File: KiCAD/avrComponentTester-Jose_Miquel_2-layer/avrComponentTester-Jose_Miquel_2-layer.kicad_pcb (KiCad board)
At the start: 2 copper layers, 17 parts, among them J4 3-pin_test_header, Q1 2N3904, Q2 2N3904, Q3 2N3906, SW1 EC11, U1 ST7735_1.8, U2 ATmega328P-PU

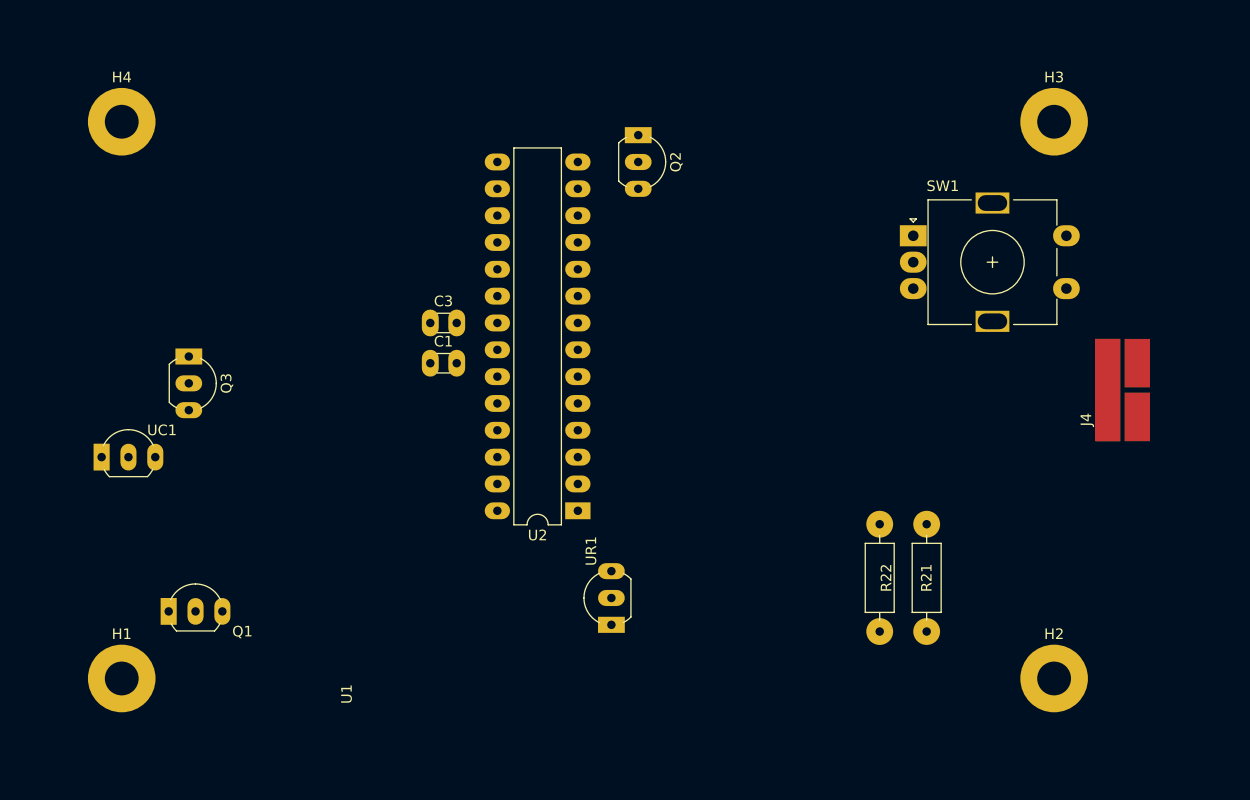
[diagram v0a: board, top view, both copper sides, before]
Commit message: kicad6
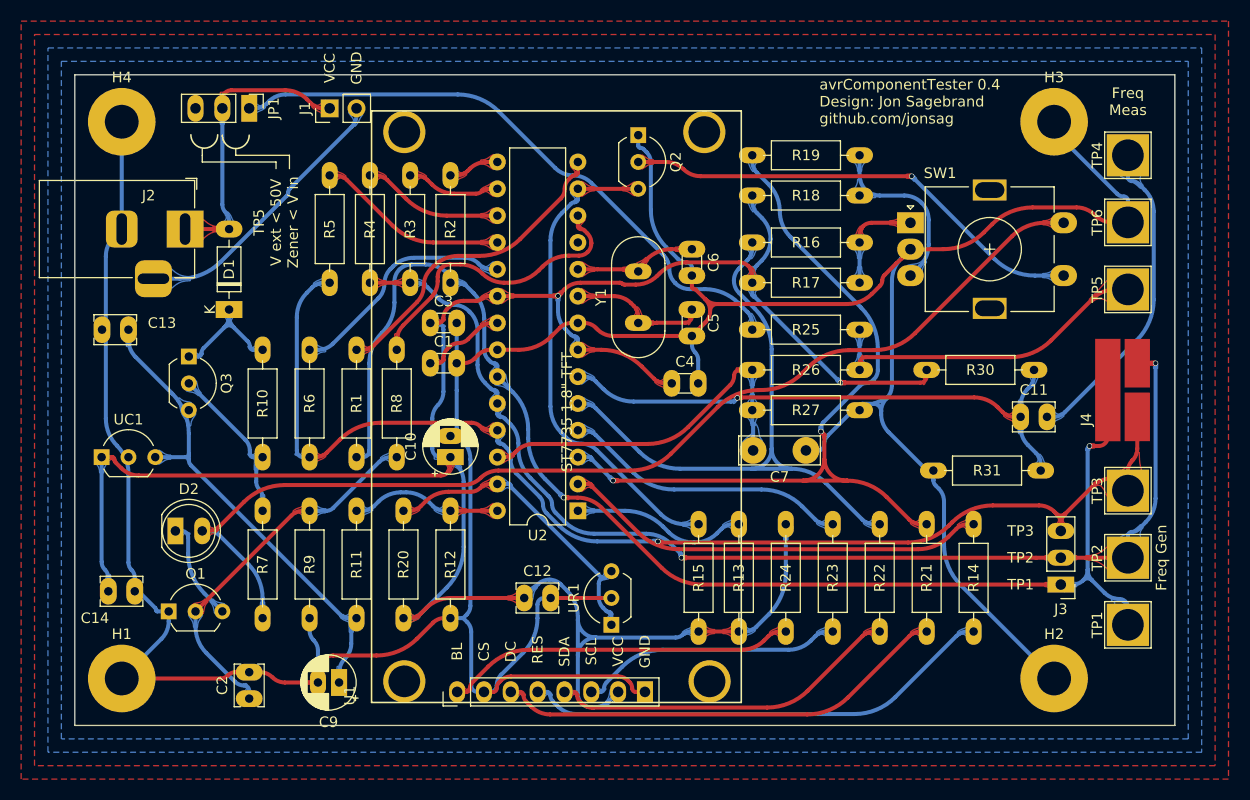
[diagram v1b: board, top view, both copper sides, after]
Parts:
- added C10: 10u, My_Misc:CP_Radial_D5.0mm_P2.00mm_larger, F.Cu at (132.7, 81.3)
- added C11: 100n, My_Misc:C_Disc_D3.8mm_W2.6mm_P2.50mm_large, F.Cu at (186.7, 77.5)
- added C12: 100n, My_Misc:C_Disc_D3.8mm_W2.6mm_P2.50mm_large, F.Cu at (139.7, 94.6)
- added C13: 100n, My_Misc:C_Disc_D3.8mm_W2.6mm_P2.50mm_large, F.Cu at (102.2, 69.2)
- added C14: 100n, My_Misc:C_Disc_D3.8mm_W2.6mm_P2.50mm_large, F.Cu at (100.3, 94.0)
- added C2: 10n, My_Misc:C_Disc_D3.8mm_W2.6mm_P2.50mm_large, F.Cu at (113.7, 104.1)
- added C4: 100n, My_Misc:C_Disc_D3.0mm_W1.6mm_P2.50mm_larg, F.Cu at (153.7, 74.3)
- added C5: 22p, My_Misc:C_Disc_D3.0mm_W1.6mm_P2.50mm_larg, F.Cu at (155.6, 67.3)
- added C6: 22p, My_Misc:C_Disc_D3.0mm_W1.6mm_P2.50mm_larg, F.Cu at (155.6, 61.6)
- added C7: 10n 100V, My_Misc:C_Disc_D7.5mm_W2.5mm_P5.00mm_larger, F.Cu at (166.4, 80.6)
- added C9: 10u, My_Misc:CP_Radial_D5.0mm_P2.00mm_larger, F.Cu at (122.2, 102.6)
- added D1: BAT43, My_Misc:D_DO-35_SOD27_P7.62mm_Horizontal_large, F.Cu at (111.8, 67.3)
- added D2: LED, My_Misc:LED_D5.0mm_larger_pads, F.Cu at (106.7, 88.3)
- added J1: 2-pin_power_input_header, My_Headers:2-pin_power_input_header, F.Cu at (121.3, 48.3)
- added J2: 8-15VDC In, My_Misc:BarrelJack_Horizontal, F.Cu at (107.6, 59.7)
- added J3: 3-pin_test_header, My_Headers:3-pin_test_header_large, F.Cu at (190.5, 93.3)
- added JP1: Vext <50V, Zener < VCC, My_Parts:Jumper_1x03_P2.54mm_large, F.Cu at (113.7, 48.3)
- added R1: 680R, My_Misc:R_Axial_DIN0207_L6.3mm_D2.5mm_P10.16mm_Horizontal_larger_pads, F.Cu at (123.8, 71.1)
- added R10: 33k, My_Misc:R_Axial_DIN0207_L6.3mm_D2.5mm_P10.16mm_Horizontal_larger_pads, F.Cu at (114.9, 81.3)
- added R11: 10k, My_Misc:R_Axial_DIN0207_L6.3mm_D2.5mm_P10.16mm_Horizontal_larger_pads, F.Cu at (123.8, 96.5)
- added R12: 3k3, My_Misc:R_Axial_DIN0207_L6.3mm_D2.5mm_P10.16mm_Horizontal_larger_pads, F.Cu at (132.7, 96.5)
- added R13: 10k, My_Misc:R_Axial_DIN0207_L6.3mm_D2.5mm_P10.16mm_Horizontal_larger_pads, F.Cu at (160.0, 97.8)
- added R14: 10k, My_Misc:R_Axial_DIN0207_L6.3mm_D2.5mm_P10.16mm_Horizontal_larger_pads, F.Cu at (182.2, 87.6)
- added R15: 27k, My_Misc:R_Axial_DIN0207_L6.3mm_D2.5mm_P10.16mm_Horizontal_larger_pads, F.Cu at (156.2, 97.8)
- added R16: 1k, My_Misc:R_Axial_DIN0207_L6.3mm_D2.5mm_P10.16mm_Horizontal_larger_pads, F.Cu at (161.3, 61.0)
- added R17: 10k, My_Misc:R_Axial_DIN0207_L6.3mm_D2.5mm_P10.16mm_Horizontal_larger_pads, F.Cu at (161.3, 64.8)
- added R18: 10k, My_Misc:R_Axial_DIN0207_L6.3mm_D2.5mm_P10.16mm_Horizontal_larger_pads, F.Cu at (161.3, 56.5)
- added R19: 1k, My_Misc:R_Axial_DIN0207_L6.3mm_D2.5mm_P10.16mm_Horizontal_larger_pads, F.Cu at (161.3, 52.7)
- added R2: 470k, My_Misc:R_Axial_DIN0207_L6.3mm_D2.5mm_P10.16mm_Horizontal_larger_pads, F.Cu at (132.7, 54.6)
- added R20: 2k2, My_Misc:R_Axial_DIN0207_L6.3mm_D2.5mm_P10.16mm_Horizontal_larger_pads, F.Cu at (128.3, 96.5)
- added R23: 10k, My_Misc:R_Axial_DIN0207_L6.3mm_D2.5mm_P10.16mm_Horizontal_larger_pads, F.Cu at (168.9, 87.6)
- added R24: 220R, My_Misc:R_Axial_DIN0207_L6.3mm_D2.5mm_P10.16mm_Horizontal_larger_pads, F.Cu at (164.5, 87.6)
- added R25: 2k2, My_Misc:R_Axial_DIN0207_L6.3mm_D2.5mm_P10.16mm_Horizontal_larger_pads, F.Cu at (171.4, 69.2)
- added R26: 179k45, My_Misc:R_Axial_DIN0207_L6.3mm_D2.5mm_P10.16mm_Horizontal_larger_pads, F.Cu at (161.3, 73.0)
- added R27: 20k, My_Misc:R_Axial_DIN0207_L6.3mm_D2.5mm_P10.16mm_Horizontal_larger_pads, F.Cu at (171.4, 76.8)
- added R3: 680R, My_Misc:R_Axial_DIN0207_L6.3mm_D2.5mm_P10.16mm_Horizontal_larger_pads, F.Cu at (128.9, 54.6)
- added R30: 10k, My_Misc:R_Axial_DIN0207_L6.3mm_D2.5mm_P10.16mm_Horizontal_larger_pads, F.Cu at (188.0, 73.0)
- added R31: 10k, My_Misc:R_Axial_DIN0207_L6.3mm_D2.5mm_P10.16mm_Horizontal_larger_pads, F.Cu at (178.4, 82.5)
- added R4: 470k, My_Misc:R_Axial_DIN0207_L6.3mm_D2.5mm_P10.16mm_Horizontal_larger_pads, F.Cu at (125.1, 54.6)
- added R5: 680R, My_Misc:R_Axial_DIN0207_L6.3mm_D2.5mm_P10.16mm_Horizontal_larger_pads, F.Cu at (121.3, 54.6)
- added R6: 470k, My_Misc:R_Axial_DIN0207_L6.3mm_D2.5mm_P10.16mm_Horizontal_larger_pads, F.Cu at (119.4, 71.1)
- added R7: 3k3, My_Misc:R_Axial_DIN0207_L6.3mm_D2.5mm_P10.16mm_Horizontal_larger_pads, F.Cu at (114.9, 96.5)
- added R8: 27k, My_Misc:R_Axial_DIN0207_L6.3mm_D2.5mm_P10.16mm_Horizontal_larger_pads, F.Cu at (127.6, 81.3)
- added R9: 100k, My_Misc:R_Axial_DIN0207_L6.3mm_D2.5mm_P10.16mm_Horizontal_larger_pads, F.Cu at (119.4, 86.4)
- added TP1: TestPoint, My_Parts:TestPoint_THTPad_4.0x4.0mm_Drill3.0mm, F.Cu at (196.8, 97.2)
- added TP2: TestPoint, My_Parts:TestPoint_THTPad_4.0x4.0mm_Drill3.0mm, F.Cu at (196.8, 90.8)
- added TP3: TestPoint, My_Parts:TestPoint_THTPad_4.0x4.0mm_Drill3.0mm, F.Cu at (196.8, 84.5)
- added TP4: TestPoint, My_Parts:TestPoint_THTPad_4.0x4.0mm_Drill3.0mm, F.Cu at (196.8, 52.7)
- added TP5: TestPoint, My_Parts:TestPoint_THTPad_4.0x4.0mm_Drill3.0mm, F.Cu at (196.8, 65.4)
- added TP6: TestPoint, My_Parts:TestPoint_THTPad_4.0x4.0mm_Drill3.0mm, F.Cu at (196.8, 59.1)
- added Y1: 8MHz, My_Misc:Crystal_HC49-4H_Vertical_large, F.Cu at (150.5, 68.6)
- Q1, Q2, Q3, UC1, UR1: footprint My_Misc:TO-92_Inline_Wide_large -> Package_TO_SOT_THT:TO-92_Inline_Wide
- SW1: value EC11 -> RotaryEncoder_Switch
- U1: value ST7735_1.8 -> ST7735_1.8"_TFT_128x160; footprint My_Parts:ST7735_1.8_TFT_display_128x160_no-SD_large -> My_Parts:ST7735_1.8_TFT_display_128x160_large
- U2: footprint Package_DIP:DIP-28_W7.62mm_LongPads -> Package_DIP:DIP-28_W7.62mm
- moved SW1 1.26 mm to (176.3, 59.1)
- moved U1 0.31 mm to (133.3, 103.5)
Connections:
- SW1 pad S1: Net-(D2-Pad2) -> Net-(Q2-Pad2)
- SW1 pad S2: Net-(Q2-Pad2) -> Net-(D2-Pad2)
- U2 pad 11: Net-(U2-Pad11) -> unconnected-(U2-Pad11)
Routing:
- net TPGND: track 0.00 -> 341.5 mm
- net +5V: track 0.00 -> 226.3 mm, vias 0 -> 2
- net TP1: track 0.00 -> 130.7 mm, vias 0 -> 2
- net TP3: track 0.00 -> 117.6 mm, vias 0 -> 1
- net TP2: track 0.00 -> 109.4 mm, vias 0 -> 2
- net Net-(D2-Pad2): track 0.00 -> 102.6 mm
- net A0: track 0.00 -> 77.2 mm, vias 0 -> 2
- net SDA: track 0.00 -> 59.7 mm
- net Net-(JP1-Pad1): track 0.00 -> 57.8 mm
- net FreqMeas: track 0.00 -> 53.8 mm, vias 0 -> 1
- net VREF: track 0.00 -> 47.2 mm
- net Net-(Q2-Pad3): track 0.00 -> 46.3 mm
- net Net-(R14-Pad2): track 0.00 -> 45.1 mm
- net Net-(Q2-Pad2): track 0.00 -> 44.2 mm, vias 0 -> 1
- net Net-(R21-Pad2): track 0.00 -> 43.2 mm
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- added copper zone on B.Cu, net (none)
- added copper zone on F.Cu, net (none)
- added copper zone on B.Cu, net TPGND
- added copper zone on F.Cu, net TPGND
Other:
- board outline added: 104.1 x 61.6 mm
- net class Default removed
- board text added: "Freq Gen"
- board text added: "Freq Meas"
- board text added: "TP5 V ext < 50V Zener < V in"
- board text added: "avrComponentTester 0.4 Design: Jon Sagebrand github.com/jonsag"
